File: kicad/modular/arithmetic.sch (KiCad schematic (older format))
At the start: 31 parts, among them J4 Header, J5 DIFFX, J6 DIFFY, J7 SUM, U5 OPA197, U6 OPA2197

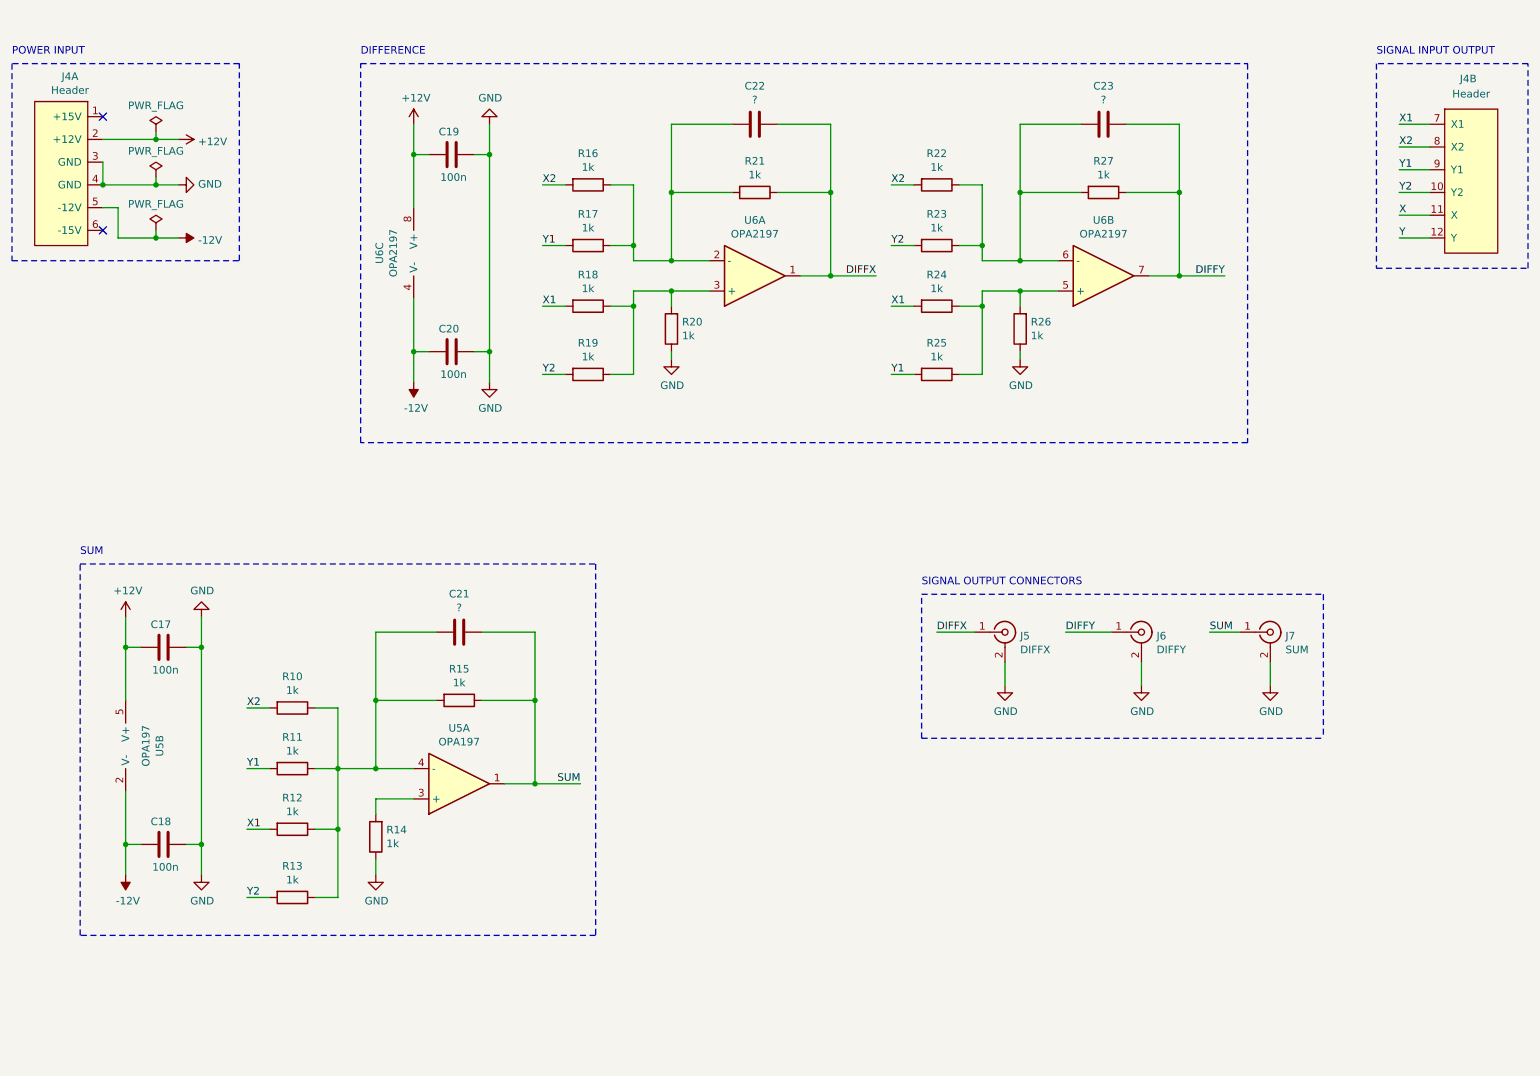
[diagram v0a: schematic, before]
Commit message: added pcb design of arithmetic board
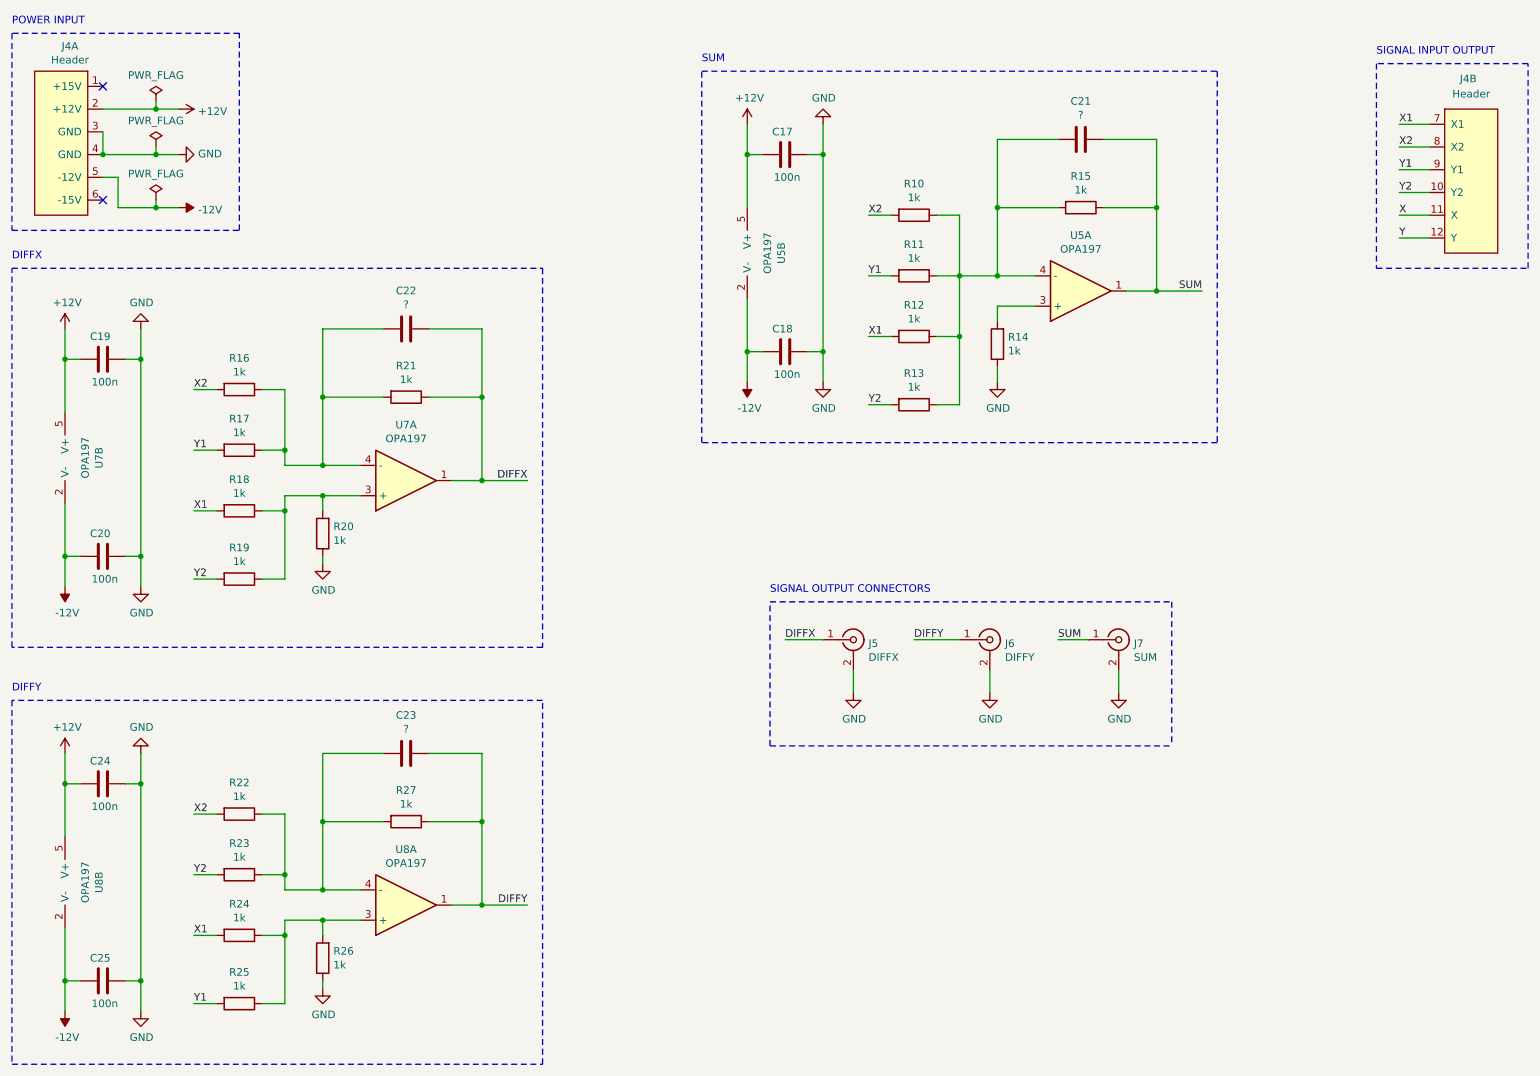
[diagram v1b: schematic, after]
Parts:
- removed U6: OPA2197, Connector_Coaxial:SMA_Amphenol_901-144_Vertical, symbol Device:Opamp_Dual_Generic
- added C24, C25: 100n, Capacitor_SMD:C_0603_1608Metric, symbol Device:C
- added U7, U8: OPA197, OPA197IDR:SOIC127P600X175-8N, symbol Device:Opamp_Generic
- U5: footprint Connector_Coaxial:SMA_Amphenol_901-144_Vertical -> OPA197IDR:SOIC127P600X175-8N
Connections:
- net +12V: now also C24.1, U7.5 (V+), U8.5 (V+)
- net -12V: now also C25.1, U7.2 (V-), U8.2 (V-)
- net DIFFX: now also U7.1
- net DIFFY: now also U8.1
- net GND: now also C24.2, C25.2
- net at C22.2, R16.1, R17.1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: now also U7.4 (-)
- net at R18.1, R19.1, R20.2: now also U7.3 (+)
- net at C23.2, R22.1, R23.1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: now also U8.4 (-)
- net at R24.1, R25.1, R26.2: now also U8.3 (+)
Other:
- note added: "DIFFX"
- note added: "DIFFY"
- note removed: "DIFFERENCE"
- moved on the sheet: C17, C18, C19, C20, C21, C22, C23, J4A, J5, J6, J7, R10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
